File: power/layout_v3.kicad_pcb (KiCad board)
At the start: 2 copper layers, 9 parts

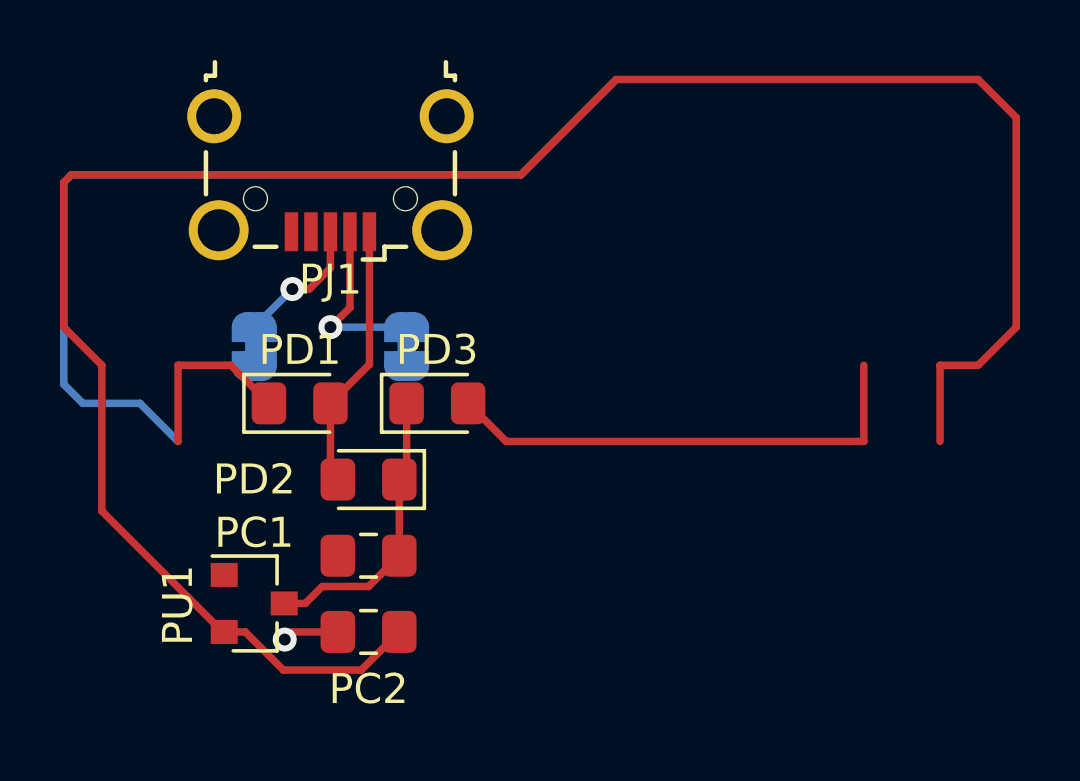
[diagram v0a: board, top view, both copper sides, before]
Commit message: WIP STM32{F,L}xxxCxTx layout
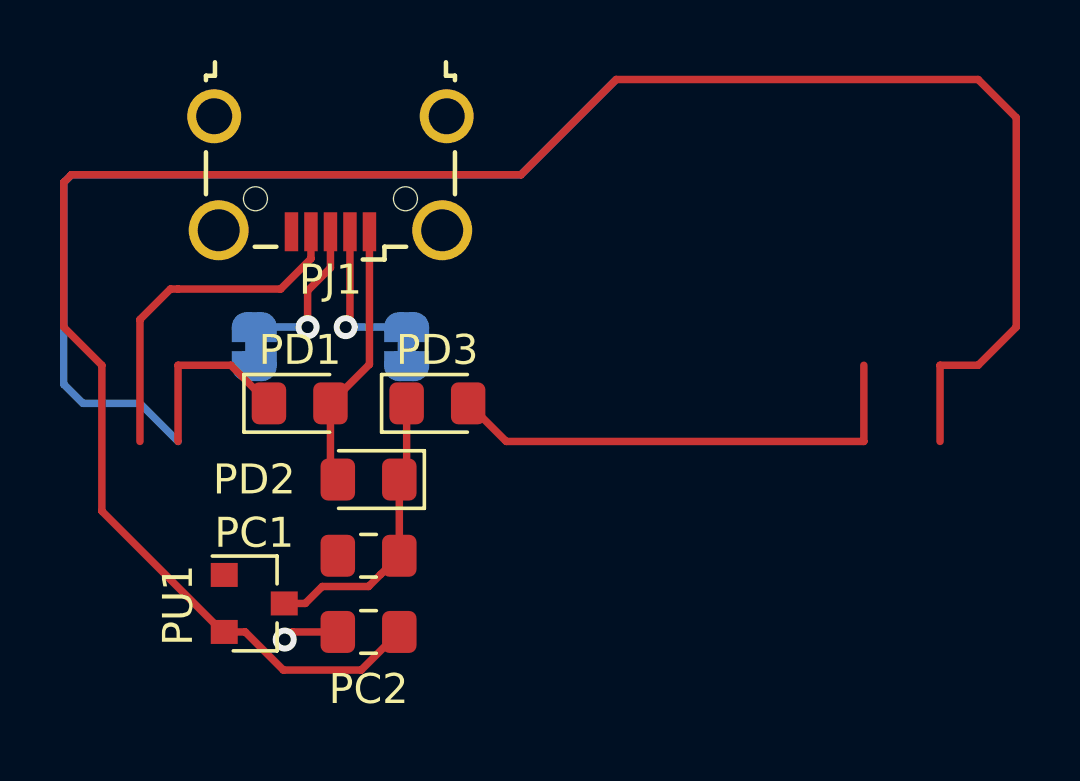
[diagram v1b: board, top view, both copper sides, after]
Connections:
- net +5V renamed 5V
- PD3 pad 2: (no net) -> VBAT
- PJ1 pad 4: (no net) -> Net-(PJ1-Pad4)
- PSJ1 pad 2: (no net) -> USB_D+
- PSJ2 pad 2: (no net) -> USB_D-
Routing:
- net +5V: track 0.00 -> 31.2 mm
- net 5V: track 37.3 -> 6.10 mm
- net VBAT: track 0.00 -> 16.3 mm
- net (no net): track 16.3 -> 0.00 mm
- net Net-(PJ1-Pad4): track 0.00 -> 11.5 mm
- net Net-(PJ1-Pad2): track 5.99 -> 5.27 mm
- net Net-(PJ1-Pad3): track 4.56 -> 5.27 mm
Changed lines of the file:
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@@
     (thickness 1.6)
     (drawings 16)
-    (tracks 56)
+    (tracks 61)
     (zones 0)
     (modules 9)
-    (nets 8)
+    (nets 13)
   )
   (page A4)
@@
   (net 6 "Net-(PJ1-Pad2)")
   (net 7 +5V)
+  (net 8 5V)
+  (net 9 VBAT)
+  (net 10 "Net-(PJ1-Pad4)")
+  (net 11 USB_D+)
+  (net 12 USB_D-)
   (net_class Default "Dit is de standaard class."
     (clearance 0.2)
@@
     (uvia_drill 0.1)
     (add_net +5V)
+    (add_net 5V)
     (add_net GND)
     (add_net "Net-(PJ1-Pad2)")
     (add_net "Net-(PJ1-Pad3)")
+    (add_net "Net-(PJ1-Pad4)")
+    (add_net USB_D+)
+    (add_net USB_D-)
+    (add_net VBAT)
     (add_net VBUS)
     (add_net VDD)
@@
       ))
     (pad 2 smd custom (at 0.65 0 270) (size 1 0.5) (layers B.Cu B.Mask)
-      (zone_connect 2)
+      (net 12 USB_D-) (zone_connect 2)
       (options (clearance outline) (anchor rect))
       (primitives
@@
       ))
     (pad 2 smd custom (at 0.65 0 270) (size 1 0.5) (layers B.Cu B.Mask)
-      (zone_connect 2)
+      (net 11 USB_D+) (zone_connect 2)
       (options (clearance outline) (anchor rect))
       (primitives
@@
     (pad 5 smd rect (at 1.3 -1.9 180) (size 0.45 1.3) (layers F.Cu F.Paste F.Mask)
       (net 1 GND))
-    (pad 4 smd rect (at 0.65 -1.9 180) (size 0.45 1.3) (layers F.Cu F.Paste F.Mask))
+    (pad 4 smd rect (at 0.65 -1.9 180) (size 0.45 1.3) (layers F.Cu F.Paste F.Mask)
+      (net 10 "Net-(PJ1-Pad4)"))
     (pad 3 smd rect (at 0 -1.9 180) (size 0.45 1.3) (layers F.Cu F.Paste F.Mask)
       (net 5 "Net-(PJ1-Pad3)"))
@@
     (fp_line (start -0.7 -0.6) (end -1 -0.3) (layer F.Fab) (width 0.1))
     (fp_line (start 1 -0.6) (end -0.7 -0.6) (layer F.Fab) (width 0.1))
-    (pad 2 smd roundrect (at 1.025 0) (size 1.15 1.4) (layers F.Cu F.Paste F.Mask) (roundrect_rratio 0.217391))
+    (pad 2 smd roundrect (at 1.025 0) (size 1.15 1.4) (layers F.Cu F.Paste F.Mask) (roundrect_rratio 0.217391)
+      (net 9 VBAT))
     (pad 1 smd roundrect (at -1.025 0) (size 1.15 1.4) (layers F.Cu F.Paste F.Mask) (roundrect_rratio 0.217391)
       (net 2 VREG_IN))
@@
       (net 4 VBUS))
     (pad 1 smd roundrect (at -1.025 0) (size 1.15 1.4) (layers F.Cu F.Paste F.Mask) (roundrect_rratio 0.217391)
-      (net 7 +5V))
+      (net 8 5V))
     (model ${KISYS3DMOD}/Diode_SMD.3dshapes/D_0805_2012Metric.wrl
       (at (xyz 0 0 0))
@@
   (gr_line (start 132.08 109.22) (end 170.18 109.22) (layer Dwgs.User) (width 0.05))
   (gr_line (start 132.08 50.8) (end 132.08 109.22) (layer Dwgs.User) (width 0.05))
-  (segment (start 162.56 60.96) (end 162.56 63.5) (width 0.25) (layer F.Cu) (net 0))
-  (segment (start 150.64 63.5) (end 149.37 62.23) (width 0.25) (layer F.Cu) (net 0))
-  (segment (start 162.56 63.5) (end 150.64 63.5) (width 0.25) (layer F.Cu) (net 0))
+  (segment (start 162.56 60.96) (end 162.56 63.5) (width 0.25) (layer F.Cu) (net 9))
+  (segment (start 150.64 63.5) (end 149.37 62.23) (width 0.25) (layer F.Cu) (net 9))
+  (segment (start 162.56 63.5) (end 150.64 63.5) (width 0.25) (layer F.Cu) (net 9))
   (via (at 143.256 70.104) (size 0.8) (drill 0.4) (layers F.Cu B.Cu) (net 1))
   (segment (start 145.025 69.85) (end 143.51 69.85) (width 0.25) (layer F.Cu) (net 1))
@@
   (segment (start 146.08 60.93) (end 146.08 56.51) (width 0.25) (layer F.Cu) (net 4))
   (segment (start 144.78 62.23) (end 146.08 60.93) (width 0.25) (layer F.Cu) (net 4))
-  (via (at 143.51 58.42) (size 0.8) (drill 0.4) (layers F.Cu B.Cu) (net 5))
-  (segment (start 142.24 59.69) (end 143.51 58.42) (width 0.25) (layer B.Cu) (net 5))
-  (segment (start 144.78 57.41) (end 144.78 56.51) (width 0.25) (layer F.Cu) (net 5))
-  (segment (start 144.075685 58.42) (end 144.78 57.715685) (width 0.25) (layer F.Cu) (net 5))
-  (segment (start 144.78 57.715685) (end 144.78 57.41) (width 0.25) (layer F.Cu) (net 5))
-  (segment (start 143.51 58.42) (end 144.075685 58.42) (width 0.25) (layer F.Cu) (net 5))
-  (via (at 144.78 59.69) (size 0.8) (drill 0.4) (layers F.Cu B.Cu) (net 6))
-  (segment (start 145.43 56.51) (end 145.43 59.04) (width 0.25) (layer F.Cu) (net 6))
-  (segment (start 145.43 59.04) (end 144.78 59.69) (width 0.25) (layer F.Cu) (net 6))
-  (segment (start 144.78 59.69) (end 147.32 59.69) (width 0.25) (layer B.Cu) (net 6))
-  (segment (start 141.46 60.96) (end 142.73 62.23) (width 0.25) (layer F.Cu) (net 7))
-  (segment (start 139.7 60.96) (end 141.46 60.96) (width 0.25) (layer F.Cu) (net 7))
-  (segment (start 139.7 60.96) (end 139.7 63.5) (width 0.25) (layer F.Cu) (net 7))
+  (via (at 144.018 59.69) (size 0.8) (drill 0.4) (layers F.Cu B.Cu) (net 5))
+  (segment (start 144.018 58.477685) (end 144.018 59.69) (width 0.25) (layer F.Cu) (net 5))
+  (segment (start 144.78 56.51) (end 144.78 57.715685) (width 0.25) (layer F.Cu) (net 5))
+  (segment (start 144.78 57.715685) (end 144.018 58.477685) (width 0.25) (layer F.Cu) (net 5))
+  (segment (start 144.018 59.69) (end 142.24 59.69) (width 0.25) (layer B.Cu) (net 5))
+  (via (at 145.288 59.69) (size 0.8) (drill 0.4) (layers F.Cu B.Cu) (net 6))
+  (segment (start 147.32 59.69) (end 145.288 59.69) (width 0.25) (layer B.Cu) (net 6))
+  (segment (start 145.43 59.548) (end 145.288 59.69) (width 0.25) (layer F.Cu) (net 6))
+  (segment (start 145.43 56.51) (end 145.43 59.548) (width 0.25) (layer F.Cu) (net 6))
+  (segment (start 141.46 60.96) (end 142.73 62.23) (width 0.25) (layer F.Cu) (net 8))
+  (segment (start 139.7 60.96) (end 141.46 60.96) (width 0.25) (layer F.Cu) (net 8))
+  (segment (start 139.7 60.96) (end 139.7 63.5) (width 0.25) (layer F.Cu) (net 8))
   (segment (start 151.13 54.61) (end 154.305 51.435) (width 0.25) (layer B.Cu) (net 7))
   (segment (start 138.43 62.23) (end 136.525 62.23) (width 0.25) (layer B.Cu) (net 7))
@@
   (segment (start 135.89 54.864998) (end 136.144998 54.61) (width 0.25) (layer B.Cu) (net 7))
   (segment (start 136.144998 54.61) (end 151.13 54.61) (width 0.25) (layer B.Cu) (net 7))
+  (segment (start 144.13 57.41) (end 143.12 58.42) (width 0.25) (layer F.Cu) (net 10))
+  (segment (start 144.13 56.51) (end 144.13 57.41) (width 0.25) (layer F.Cu) (net 10))
+  (segment (start 143.12 58.42) (end 139.7 58.42) (width 0.25) (layer F.Cu) (net 10))
+  (segment (start 139.7 58.42) (end 139.446 58.42) (width 0.25) (layer F.Cu) (net 10))
+  (segment (start 139.446 58.42) (end 138.43 59.436) (width 0.25) (layer F.Cu) (net 10))
+  (segment (start 138.43 59.436) (end 138.43 63.5) (width 0.25) (layer F.Cu) (net 10))
 )
